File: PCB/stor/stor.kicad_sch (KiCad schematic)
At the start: 56 parts, among them J1 Conn_01x05_Socket, J2 Conn_01x04_Socket, SW1 TS1603-TZ38HBM, SW2 TS1603-TZ38HBM, U1 STM32H723VGT6, U3 USB3300-EZK-TR, U4 TPS62177DQCR, X1 25mhz, X2 32.768k, X3 24mhz

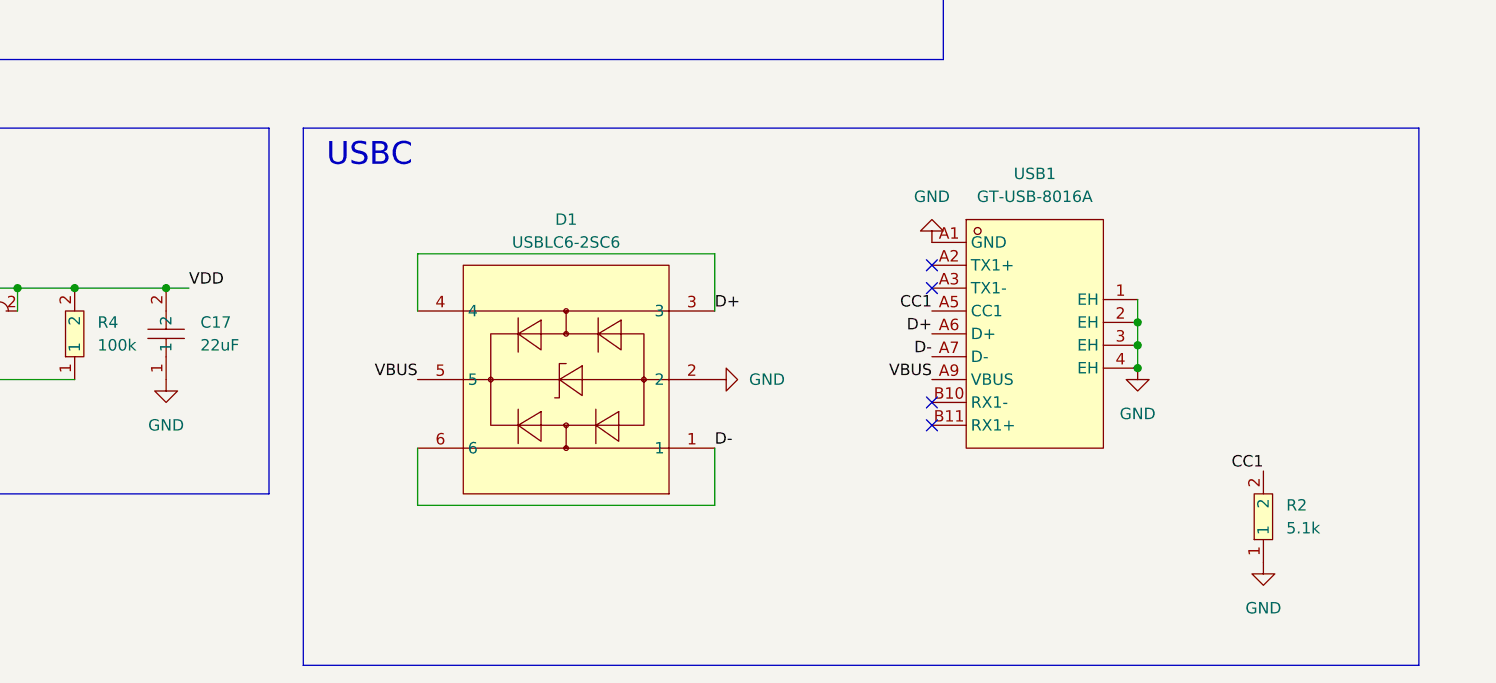
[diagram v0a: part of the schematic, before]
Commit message: new usb
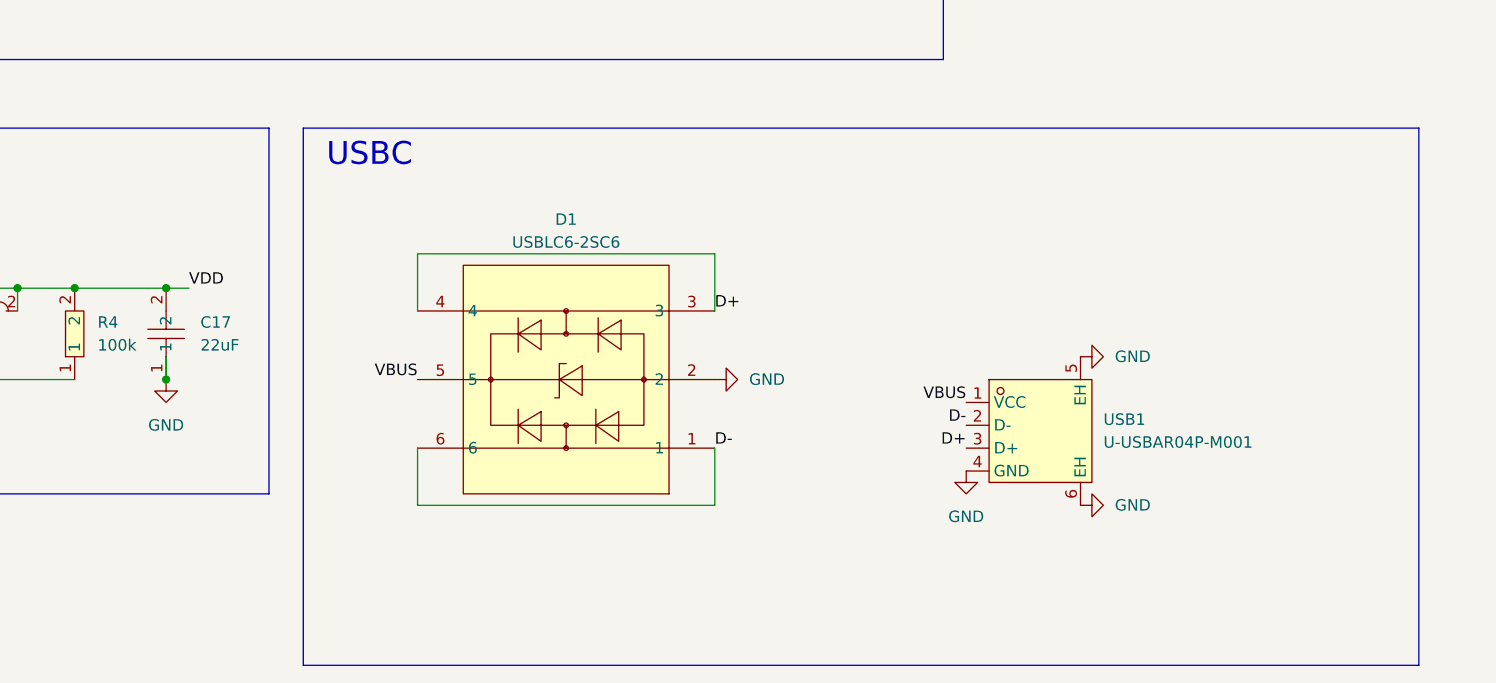
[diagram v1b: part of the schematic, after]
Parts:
- removed C17: 22uF, easyeda2kicad:C0402, symbol lcsc:HGC0402R5226M100NTEJ
- removed R2: 5.1k, easyeda2kicad:R0402, symbol easyeda2kicad:RC0402FR-075K1L
- removed USB1: GT-USB-8016A, easyeda2kicad:USB-TYPE-C-SMD_GT-USB-8016A, symbol easyeda2kicad:GT-USB-8016A
- added C17: 22uF, easyeda2kicad:C0603, symbol lcsc:CL10A226MQ8NRNC
- added USB1: U-USBAR04P-M001, easyeda2kicad:USB-SMD_KH-USB-AM-4P-CB, symbol lcsc:U-USBAR04P-M001
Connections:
- net D+: now also USB1.3 (D+)
- net D-: now also USB1.2 (D-)
- net GND: now also C17.1, USB1.4 (GND), USB1.5 (EH), USB1.6 (EH)
- net VBUS: now also USB1.1 (VCC)
- net VDD: now also C17.2
- no-connect marks 7 -> 3

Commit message: bom opt!!
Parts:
- C1, C16, C2: symbol easyeda2kicad:CL05A225KO5NQNC -> easyeda2kicad:CL05A225MQ5NSNC; LCSC Part C170151 -> C12530; MPN CL05A225KO5NQNC -> CL05A225MQ5NSNC; Manufacturer SAMSUNG(三星) -> Samsung Electro-Mechanics
- C10, C15, C18, C19, C21, C23, C26, C27, C3, C4, C5, C6, C7, C8, C9: symbol easyeda2kicad:CC0402KRX7R7BB104 -> easyeda2kicad:CL05B104KO5NNNC; LCSC Part C60474 -> C1525; MPN CC0402KRX7R7BB104 -> CL05B104KO5NNNC; Manufacturer YAGEO(国巨) -> Samsung Electro-Mechanics
- C11, C12, C13, C14, C24, C25: symbol lcsc:CC0402JRNPO9BN180 -> lcsc:0402CG180J500NT; LCSC Part C106202 -> C1549; MPN CC0402JRNPO9BN180 -> 0402CG180J500NT; Manufacturer YAGEO(国巨) -> FH
- C20, C22, C29: symbol easyeda2kicad:CL05A475KP5NRNC -> easyeda2kicad:CL05A475MP5NRNC; LCSC Part C368809 -> C23733; MPN CL05A475KP5NRNC -> CL05A475MP5NRNC; Manufacturer SAMSUNG(三星) -> Samsung Electro-Mechanics
- J1, J2: now left out of the parts list
- R1, R10, R11, R7, R8, R9: symbol easyeda2kicad:RC0402FR-0710KL -> easyeda2kicad:0402WGF1002TCE; LCSC Part C60490 -> C25744; MPN RC0402FR-0710KL -> 0402WGF1002TCE; Manufacturer YAGEO(国巨) -> UNI-ROYAL
- R4: symbol easyeda2kicad:RC0402FR-07100KL -> easyeda2kicad:0402WGF1003TCE; LCSC Part C60491 -> C25741; MPN RC0402FR-07100KL -> 0402WGF1003TCE; Manufacturer YAGEO(国巨) -> UNI-ROYAL
- R5: symbol easyeda2kicad:RC0402FR-0712KL -> easyeda2kicad:0402WGF1202TCE; LCSC Part C114760 -> C25752; MPN RC0402FR-0712KL -> 0402WGF1202TCE; Manufacturer YAGEO(国巨) -> UNI-ROYAL
- R6: symbol easyeda2kicad:RC0402FR-071ML -> easyeda2kicad:0402WGF1004TCE; LCSC Part C138033 -> C26083; MPN RC0402FR-071ML -> 0402WGF1004TCE; Manufacturer YAGEO(国巨) -> UNI-ROYAL
